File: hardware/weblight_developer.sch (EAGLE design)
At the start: 14 parts, among them U1 ATtiny85-20SU

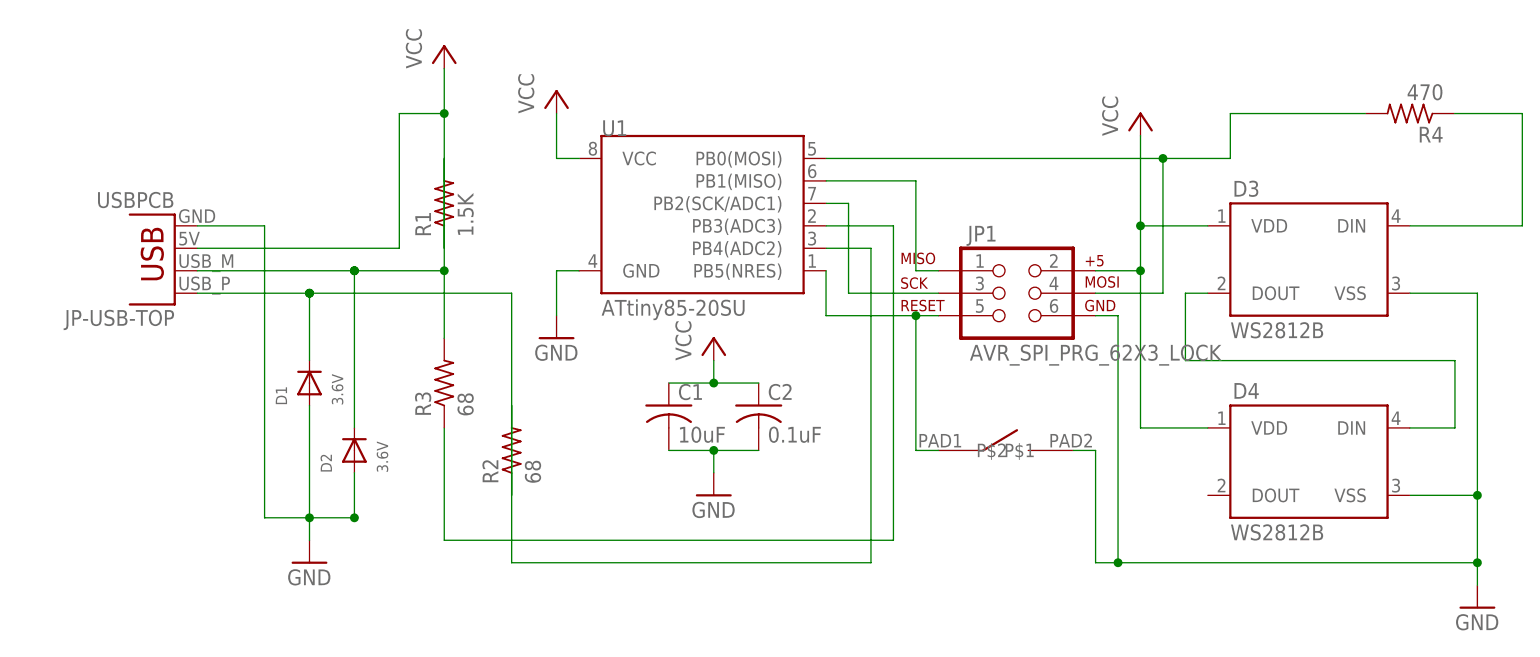
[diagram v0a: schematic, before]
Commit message: osh3 rc1
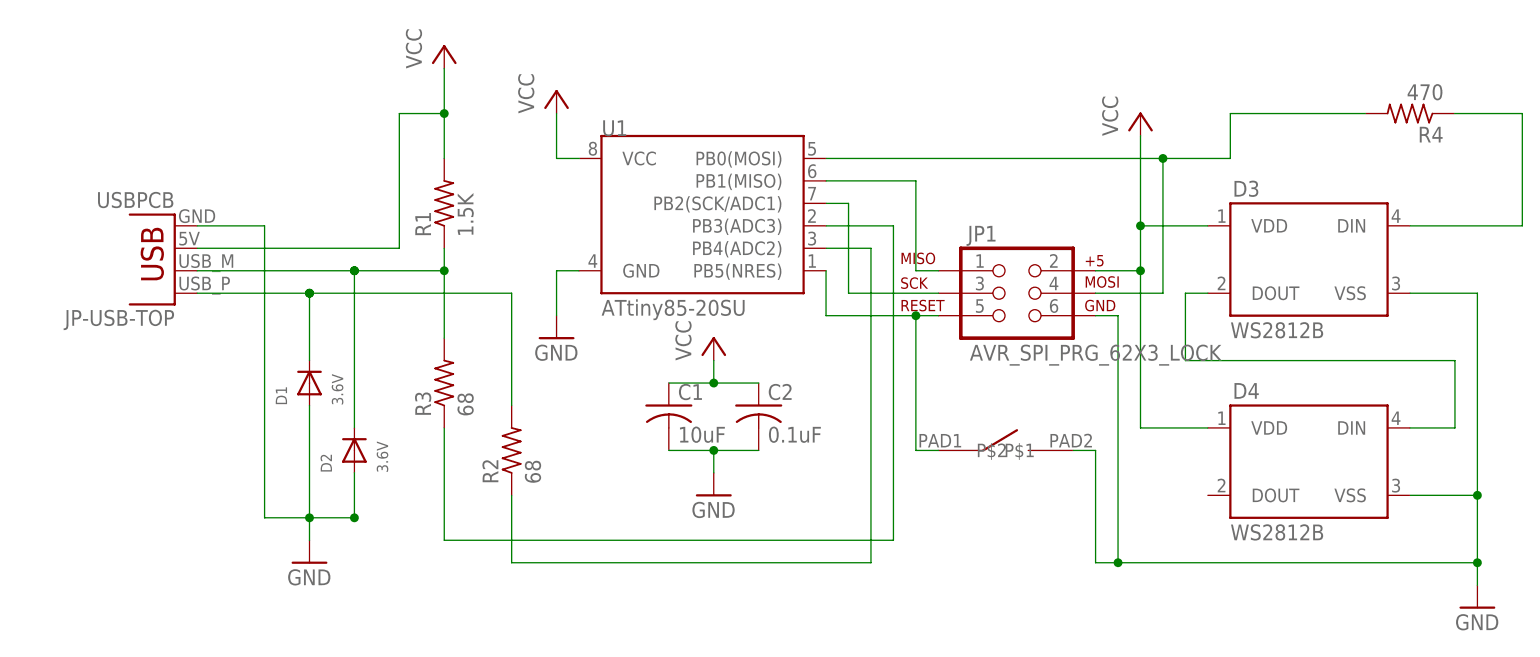
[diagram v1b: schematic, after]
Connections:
- net USB_D_MINUS_RAW: now also R1.1; no longer R1.2
- net USB_D_PLUS: now also R2.1; no longer R2.2
- net USB_D_PLUS_RAW: now also R2.2; no longer R2.1
- net VCC: now also R1.2; no longer R1.1
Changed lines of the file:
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@@
 <grid distance="0.1" unitdist="inch" unit="inch" style="lines" multiple="1" display="no" altdistance="0.01" altunitdist="inch" altunit="inch"/>
 <layers>
-<layer number="1" name="Top" color="4" fill="1" visible="yes" active="no"/>
-<layer number="16" name="Bottom" color="1" fill="1" visible="yes" active="no"/>
-<layer number="17" name="Pads" color="2" fill="1" visible="yes" active="no"/>
-<layer number="18" name="Vias" color="2" fill="1" visible="yes" active="no"/>
-<layer number="19" name="Unrouted" color="6" fill="1" visible="yes" active="no"/>
-<layer number="20" name="Dimension" color="15" fill="1" visible="yes" active="no"/>
-<layer number="21" name="tPlace" color="7" fill="1" visible="yes" active="no"/>
-<layer number="22" name="bPlace" color="7" fill="1" visible="yes" active="no"/>
-<layer number="23" name="tOrigins" color="15" fill="1" visible="yes" active="no"/>
-<layer number="24" name="bOrigins" color="15" fill="1" visible="yes" active="no"/>
-<layer number="25" name="tNames" color="7" fill="1" visible="yes" active="no"/>
-<layer number="26" name="bNames" color="7" fill="1" visible="yes" active="no"/>
-<layer number="27" name="tValues" color="7" fill="1" visible="yes" active="no"/>
-<layer number="28" name="bValues" color="7" fill="1" visible="yes" active="no"/>
+<layer number="1" name="Top" color="4" fill="1" visible="no" active="no"/>
+<layer number="16" name="Bottom" color="1" fill="1" visible="no" active="no"/>
+<layer number="17" name="Pads" color="2" fill="1" visible="no" active="no"/>
+<layer number="18" name="Vias" color="2" fill="1" visible="no" active="no"/>
+<layer number="19" name="Unrouted" color="6" fill="1" visible="no" active="no"/>
+<layer number="20" name="Dimension" color="15" fill="1" visible="no" active="no"/>
+<layer number="21" name="tPlace" color="7" fill="1" visible="no" active="no"/>
+<layer number="22" name="bPlace" color="7" fill="1" visible="no" active="no"/>
+<layer number="23" name="tOrigins" color="15" fill="1" visible="no" active="no"/>
+<layer number="24" name="bOrigins" color="15" fill="1" visible="no" active="no"/>
+<layer number="25" name="tNames" color="7" fill="1" visible="no" active="no"/>
+<layer number="26" name="bNames" color="7" fill="1" visible="no" active="no"/>
+<layer number="27" name="tValues" color="7" fill="1" visible="no" active="no"/>
+<layer number="28" name="bValues" color="7" fill="1" visible="no" active="no"/>
 <layer number="29" name="tStop" color="7" fill="3" visible="no" active="no"/>
 <layer number="30" name="bStop" color="7" fill="6" visible="no" active="no"/>
@@
 <layer number="35" name="tGlue" color="7" fill="4" visible="no" active="no"/>
 <layer number="36" name="bGlue" color="7" fill="5" visible="no" active="no"/>
-<layer number="37" name="tTest" color="7" fill="1" visible="yes" active="no"/>
-<layer number="38" name="bTest" color="7" fill="1" visible="yes" active="no"/>
+<layer number="37" name="tTest" color="7" fill="1" visible="no" active="no"/>
+<layer number="38" name="bTest" color="7" fill="1" visible="no" active="no"/>
 <layer number="39" name="tKeepout" color="4" fill="11" visible="no" active="no"/>
 <layer number="40" name="bKeepout" color="1" fill="11" visible="no" active="no"/>
@@
 <layer number="44" name="Drills" color="7" fill="1" visible="no" active="no"/>
 <layer number="45" name="Holes" color="7" fill="1" visible="no" active="no"/>
-<layer number="46" name="Milling" color="3" fill="1" visible="yes" active="no"/>
-<layer number="47" name="Measures" color="7" fill="1" visible="yes" active="no"/>
-<layer number="48" name="Document" color="7" fill="1" visible="yes" active="no"/>
-<layer number="49" name="Reference" color="7" fill="1" visible="yes" active="no"/>
-<layer number="50" name="dxf" color="7" fill="1" visible="yes" active="no"/>
-<layer number="51" name="tDocu" color="7" fill="1" visible="yes" active="no"/>
-<layer number="52" name="bDocu" color="7" fill="1" visible="yes" active="no"/>
-<layer number="53" name="tGND_GNDA" color="7" fill="9" visible="yes" active="no"/>
-<layer number="54" name="bGND_GNDA" color="1" fill="9" visible="yes" active="no"/>
-<layer number="56" name="wert" color="7" fill="1" visible="yes" active="no"/>
-<layer number="57" name="tCAD" color="7" fill="1" visible="yes" active="no"/>
-<layer number="59" name="tCarbon" color="7" fill="1" visible="yes" active="no"/>
-<layer number="60" name="bCarbon" color="7" fill="1" visible="yes" active="no"/>
+<layer number="46" name="Milling" color="3" fill="1" visible="no" active="no"/>
+<layer number="47" name="Measures" color="7" fill="1" visible="no" active="no"/>
+<layer number="48" name="Document" color="7" fill="1" visible="no" active="no"/>
+<layer number="49" name="Reference" color="7" fill="1" visible="no" active="no"/>
+<layer number="50" name="dxf" color="7" fill="1" visible="no" active="no"/>
+<layer number="51" name="tDocu" color="7" fill="1" visible="no" active="no"/>
+<layer number="52" name="bDocu" color="7" fill="1" visible="no" active="no"/>
+<layer number="53" name="tGND_GNDA" color="7" fill="9" visible="no" active="no"/>
+<layer number="54" name="bGND_GNDA" color="1" fill="9" visible="no" active="no"/>
+<layer number="56" name="wert" color="7" fill="1" visible="no" active="no"/>
+<layer number="57" name="tCAD" color="7" fill="1" visible="no" active="no"/>
+<layer number="59" name="tCarbon" color="7" fill="1" visible="no" active="no"/>
+<layer number="60" name="bCarbon" color="7" fill="1" visible="no" active="no"/>
 <layer number="90" name="Modules" color="5" fill="1" visible="yes" active="yes"/>
 <layer number="91" name="Nets" color="2" fill="1" visible="yes" active="yes"/>
@@
 <pinref part="JP-USB-TOP" gate="G$1" pin="VBUS"/>
 <wire x1="-45.72" y1="71.12" x2="-22.86" y2="71.12" width="0.1524" layer="91"/>
-<pinref part="R1" gate="G$1" pin="1"/>
+<pinref part="R1" gate="G$1" pin="2"/>
 <wire x1="-17.78" y1="86.36" x2="-22.86" y2="86.36" width="0.1524" layer="91"/>
 <junction x="-17.78" y="86.36"/>
 <pinref part="P+2" gate="VCC" pin="VCC"/>
 <wire x1="-17.78" y1="86.36" x2="-17.78" y2="91.44" width="0.1524" layer="91"/>
-<wire x1="-17.78" y1="71.12" x2="-17.78" y2="86.36" width="0.1524" layer="91"/>
+<wire x1="-17.78" y1="81.28" x2="-17.78" y2="86.36" width="0.1524" layer="91"/>
 <wire x1="-22.86" y1="71.12" x2="-22.86" y2="86.36" width="0.1524" layer="91"/>
 </segment>
@@
 <wire x1="-17.78" y1="60.96" x2="-17.78" y2="68.58" width="0.1524" layer="91"/>
 <pinref part="JP-USB-TOP" gate="G$1" pin="D-"/>
-<pinref part="R1" gate="G$1" pin="2"/>
+<pinref part="R1" gate="G$1" pin="1"/>
 <wire x1="-17.78" y1="68.58" x2="-27.94" y2="68.58" width="0.1524" layer="91"/>
 <wire x1="-27.94" y1="68.58" x2="-45.72" y2="68.58" width="0.1524" layer="91"/>
-<wire x1="-17.78" y1="81.28" x2="-17.78" y2="68.58" width="0.1524" layer="91"/>
+<wire x1="-17.78" y1="71.12" x2="-17.78" y2="68.58" width="0.1524" layer="91"/>
 <junction x="-17.78" y="68.58"/>
 <pinref part="D2" gate="G$1" pin="C"/>
@@
 <wire x1="-45.72" y1="66.04" x2="-33.02" y2="66.04" width="0.1524" layer="91"/>
 <wire x1="-33.02" y1="66.04" x2="-10.16" y2="66.04" width="0.1524" layer="91"/>
-<pinref part="R2" gate="G$1" pin="1"/>
-<wire x1="-10.16" y1="66.04" x2="-10.16" y2="43.18" width="0.1524" layer="91"/>
+<pinref part="R2" gate="G$1" pin="2"/>
+<wire x1="-10.16" y1="66.04" x2="-10.16" y2="53.34" width="0.1524" layer="91"/>
 <pinref part="D1" gate="G$1" pin="C"/>
 <wire x1="-33.02" y1="58.42" x2="-33.02" y2="66.04" width="0.1524" layer="91"/>
@@
 <net name="USB_D_PLUS" class="0">
 <segment>
-<pinref part="R2" gate="G$1" pin="2"/>
-<wire x1="-10.16" y1="53.34" x2="-10.16" y2="35.56" width="0.1524" layer="91"/>
+<pinref part="R2" gate="G$1" pin="1"/>
+<wire x1="-10.16" y1="43.18" x2="-10.16" y2="35.56" width="0.1524" layer="91"/>
 <wire x1="-10.16" y1="35.56" x2="30.48" y2="35.56" width="0.1524" layer="91"/>
 <wire x1="30.48" y1="35.56" x2="30.48" y2="71.12" width="0.1524" layer="91"/>
